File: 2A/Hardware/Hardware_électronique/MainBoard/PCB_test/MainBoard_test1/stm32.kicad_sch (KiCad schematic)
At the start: 82 parts, among them J2 Conn_ST_STDC14, SW1 SW_Push, SW2 SW_Push, SW3 SW_Push, SW4 SW_Push, U1 STM32H735IGTx, U4 AZ1117-3.3

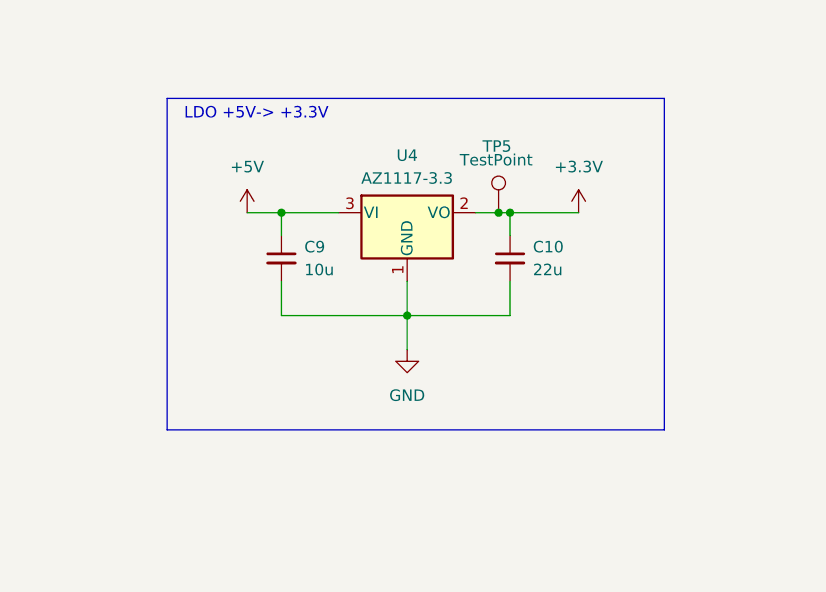
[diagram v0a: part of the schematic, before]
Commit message: pcb edits
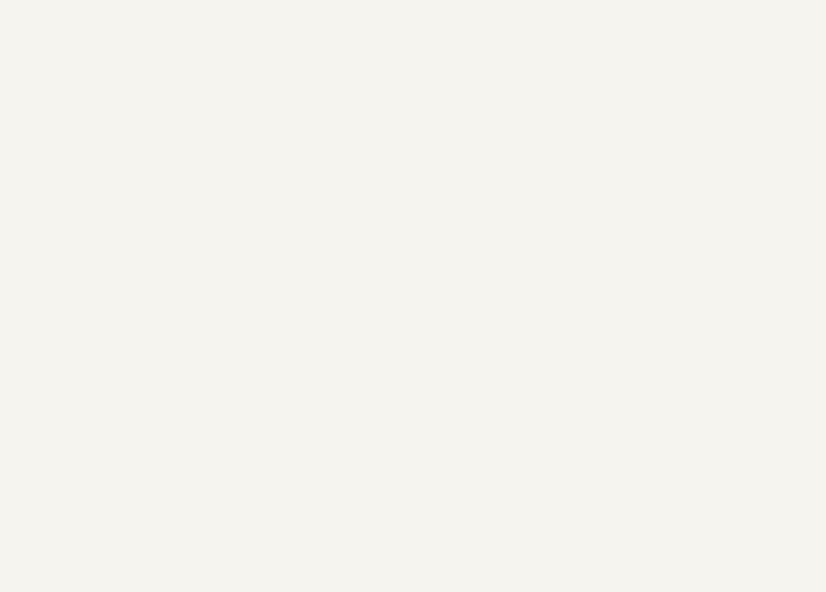
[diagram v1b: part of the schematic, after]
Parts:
- removed C10: 22u, Capacitor_SMD:C_0805_2012Metric, symbol Device:C_Small
- removed C9: 10u, Capacitor_SMD:C_0805_2012Metric, symbol Device:C_Small
- removed TP5: TestPoint, TestPoint:TestPoint_Pad_D2.0mm, symbol Connector:TestPoint
- removed U4: AZ1117-3.3, Package_TO_SOT_SMD:SOT-223-3_TabPin2, symbol Regulator_Linear:AZ1117-3.3
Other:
- note removed: "LDO +5V-> +3.3V"
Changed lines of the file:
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@@
 (kicad_sch
-	(version 20231120)
+	(version 20250114)
 	(generator "eeschema")
-	(generator_version "8.0")
+	(generator_version "9.0")
 	(paper "A2")
